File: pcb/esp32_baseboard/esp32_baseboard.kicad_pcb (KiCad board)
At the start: 2 copper layers, 175 x 175 mm, 38 parts, among them J1 Screw_12V_IN, J10 LIM_MIN_NC, J11 LIM_MAX_NC, J12 LIM_MIN_NC, J13 LIM_MAX_NC, J14 BUP_30S, J15 BUZZER_5V, J16 AOD4184, J17 TFT_TOUCH, J2 NEMA17_OUT, J4 OPTO_FIELD_IN, J5 GA12_N20, J6 GA12_N20, J7 GA12_N20, J8 LIM_MIN_NC, J9 LIM_MAX_NC, U1 ESP32_S3_DevKitC_1, U2 MP1584_5V3A, U3 TMC2209, U4 PC817_4CH, U5 DRV8871_Module, U6 DRV8871_Module, U7 DRV8871_Module, U8 MP1584_BLW, U9 PC817_4CH

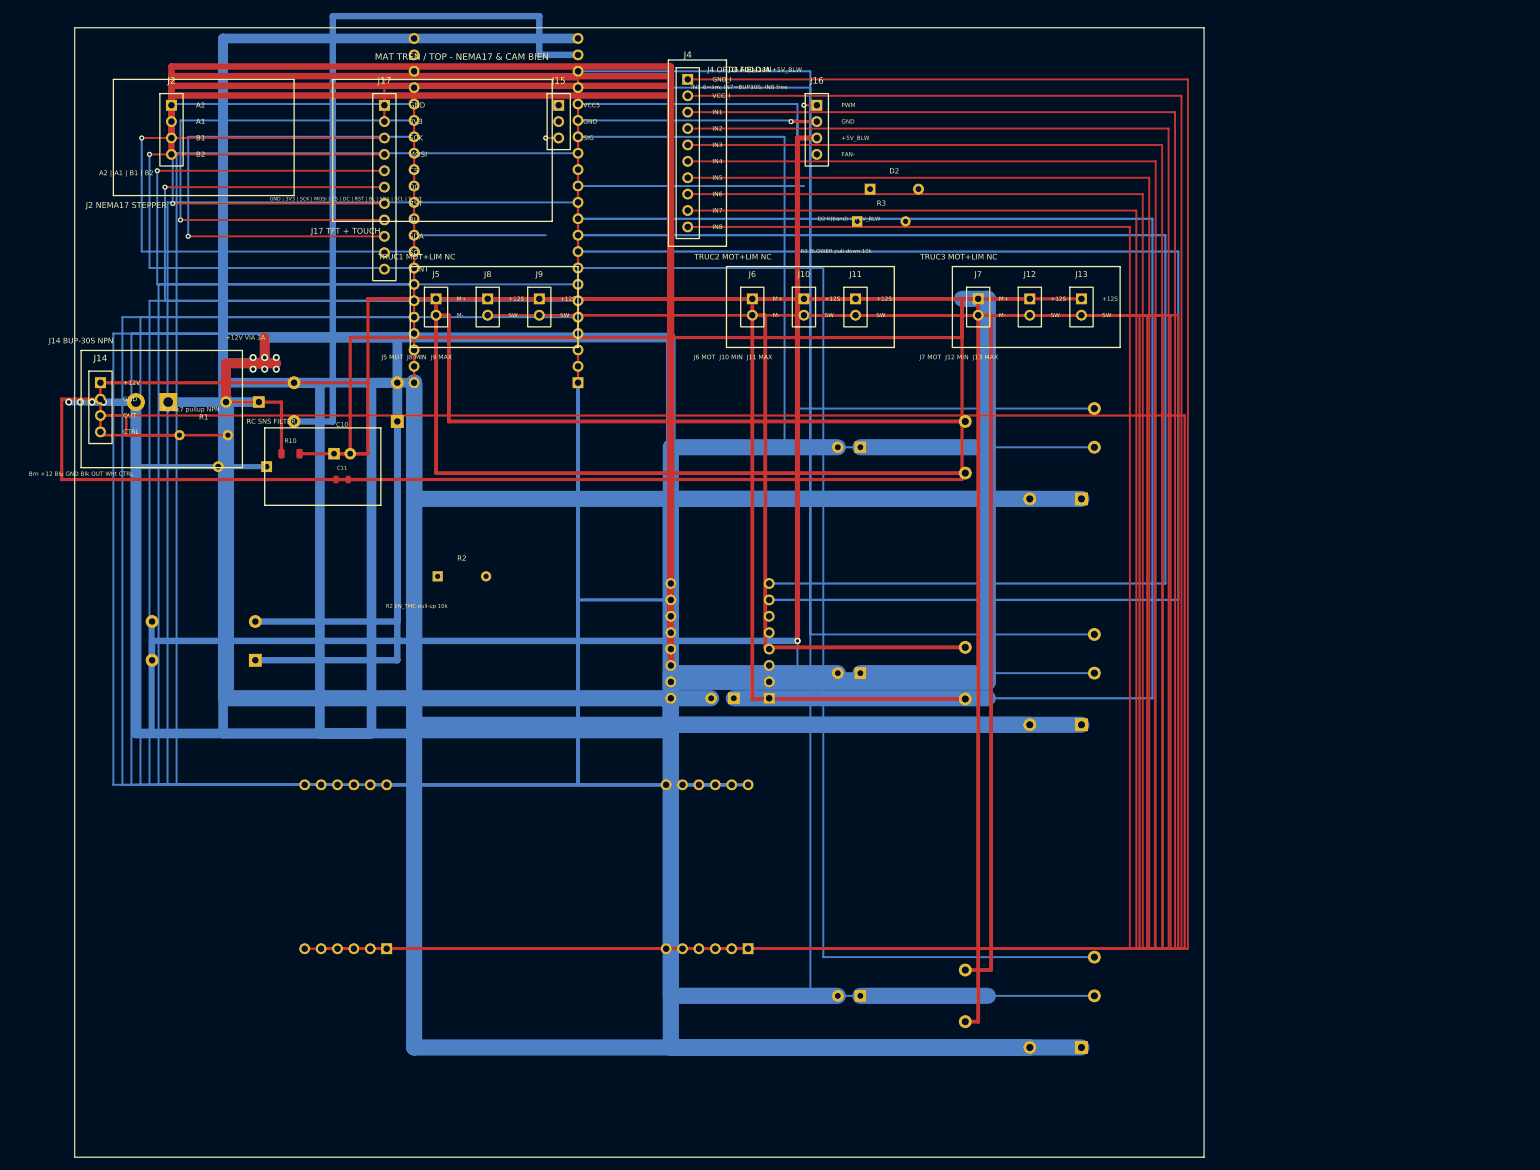
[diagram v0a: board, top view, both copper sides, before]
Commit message: sửa lỗi ngắn mạch trên board
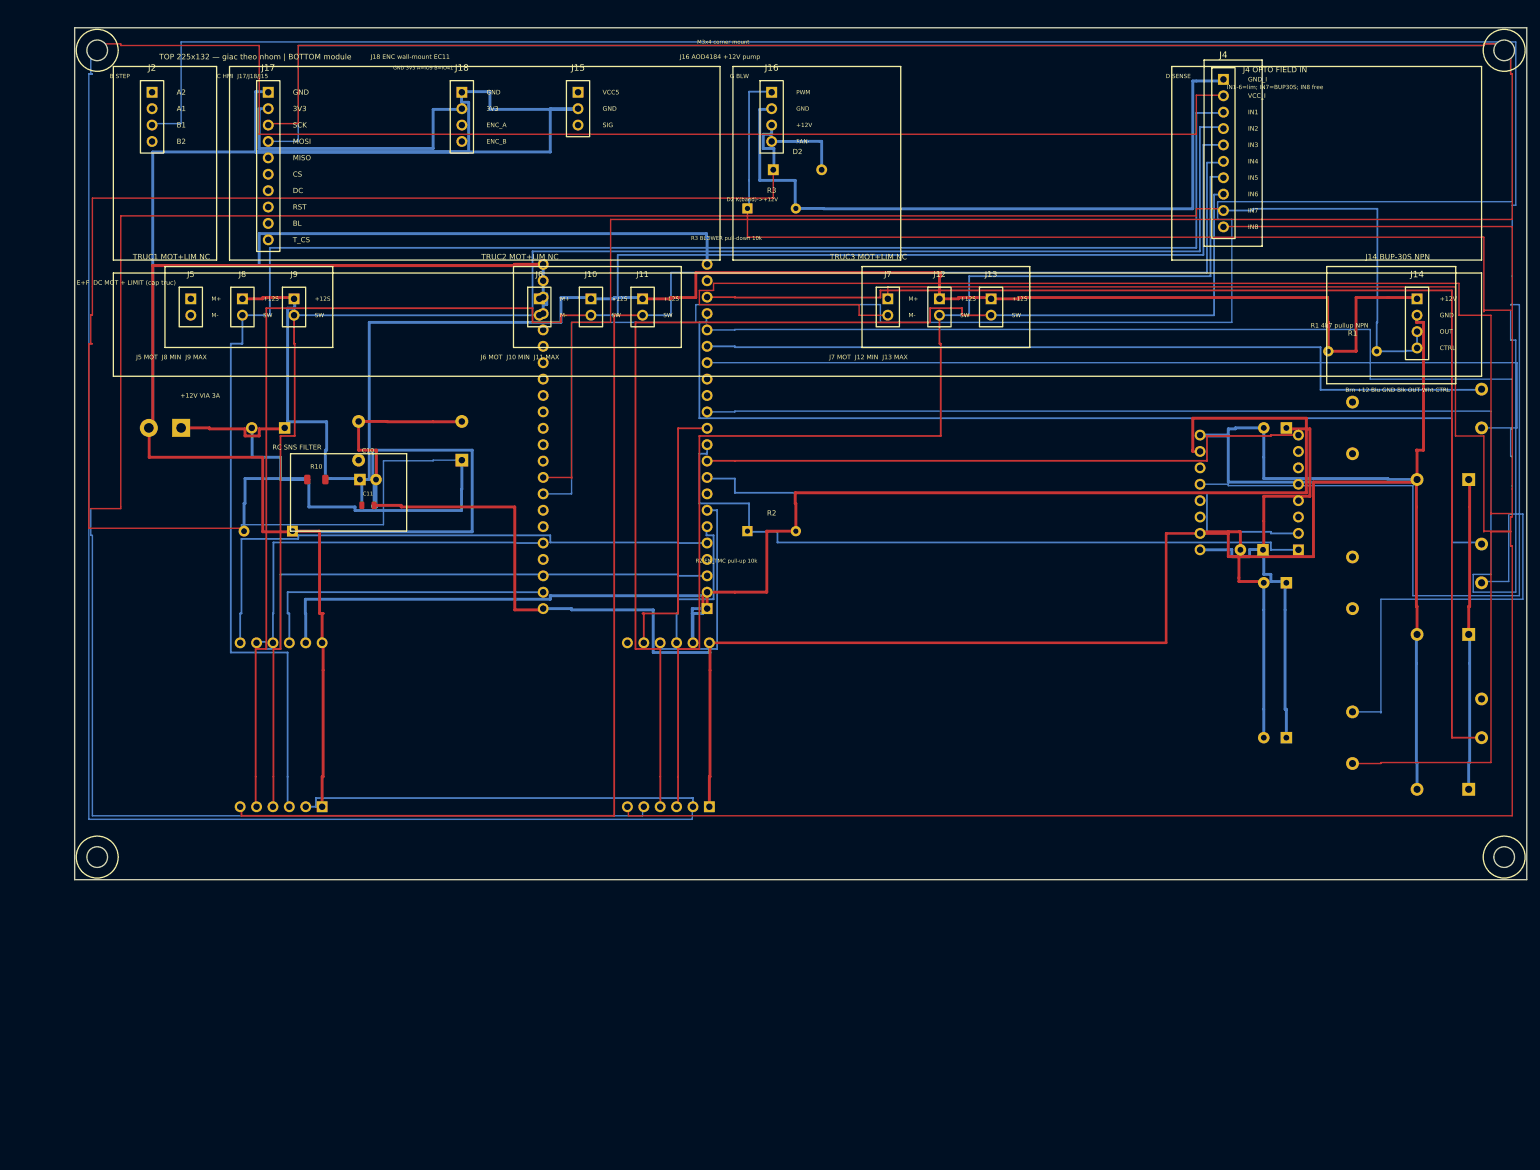
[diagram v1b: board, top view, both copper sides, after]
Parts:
- removed U8: MP1584_BLW, ESP32_Carrier:MP1584_5V3A
- added H1: M3, ESP32_Carrier:MountingHole_M3, F.Cu at (38.5, 33.5)
- added H2: M3, ESP32_Carrier:MountingHole_M3, F.Cu at (256.5, 33.5)
- added H3: M3, ESP32_Carrier:MountingHole_M3, F.Cu at (38.5, 158.5)
- added H4: M3, ESP32_Carrier:MountingHole_M3, F.Cu at (256.5, 158.5)
- added J18: EC11_ENC, ESP32_Carrier:PinHeader_1x04_ENC, F.Cu at (95.0, 40.0)
- J17: footprint ESP32_Carrier:PinHeader_1x11_TFT -> ESP32_Carrier:PinHeader_1x10_TFT
- moved J14 204.4 mm to (243.0, 72.0)
- moved R1 178.5 mm to (233.0, 80.1)
- moved U3 85.2 mm to (217.0, 102.0)
- moved C20 85.2 mm to (217.4, 110.9)
- moved J4 83.0 mm to (213.0, 38.0)
- moved C23 77.2 mm to (221.0, 140.0)
- moved U7 72.1 mm to (243.0, 140.0)
- moved C22 67.5 mm to (221.0, 116.0)
- moved C21 66.1 mm to (221.0, 92.0)
- moved U6 61.6 mm to (243.0, 116.0)
- moved U5 60.1 mm to (243.0, 92.0)
- moved R2 48.5 mm to (143.0, 108.0)
- moved U1 40.3 mm to (133.0, 120.0)
- moved J5 38.0 mm to (53.0, 72.0)
- moved J8 38.0 mm to (61.0, 72.0)
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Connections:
- net /I2C_SCL renamed /T_CS
- D2 pad 1: +5V_BLW -> +12V
- J16 pad 3: +5V_BLW -> +12V
- J17 pad 5: /TFT_CS -> /TFT_MISO
- J17 pad 6: /TFT_DC -> /TFT_CS
- J17 pad 7: /TFT_RST -> /TFT_DC
- J17 pad 8: /TFT_BL -> /TFT_RST
- J17 pad 9: /I2C_SDA -> /TFT_BL
- U1 pad 15: /OPTO_OUT8 -> /ENC_A
- U1 pad 29: /TP_INT -> /ENC_B
- U1 pad 39: /I2C_SDA -> /TFT_MISO
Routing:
- net GND: track 2326.1 -> 1179.7 mm, vias 5 -> 0
- net +12V: track 866.3 -> 435.4 mm, vias 6 -> 0
- net /OPTO_IN2: track 655.4 -> 253.0 mm, vias 1 -> 0
- net /OPTO_IN1: track 665.2 -> 270.5 mm, vias 1 -> 0
- net /OPTO_IN3: track 612.5 -> 257.1 mm, vias 1 -> 0
- net /OPTO_IN4: track 602.7 -> 255.2 mm, vias 1 -> 0
- net /TFT_MOSI: track 95.0 -> 437.6 mm, vias 1 -> 0
- net /TFT_SCK: track 97.4 -> 423.0 mm, vias 1 -> 0
- net /BLOWER: track 37.0 -> 359.9 mm, vias 1 -> 0
- net /OPTO_IN5: track 441.5 -> 182.9 mm, vias 1 -> 0
- net /OPTO_IN6: track 431.6 -> 192.1 mm, vias 1 -> 0
- net /OPTO_OUT8: track 235.9 -> 0.00 mm
- net +12V_SNS: track 487.6 -> 273.2 mm
- net /MotB1: track 170.2 -> 378.9 mm
- net /OPTO_OUT5: track 229.1 -> 24.9 mm
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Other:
- board size 175 x 175 mm -> 225 x 132 mm
- board text added: "1 POWER J1/U2"
- board text added: "2 MCU U1"
- board text added: "3 TMC"
- board text added: "B STEP"
- board text added: "B.Cu bus"
- board text added: "BOTTOM — 1 POWER | 2 MCU | 3 TMC | 4 OPTO | 5 DRV"
- board text added: "C HMI J17/J18/J15"
- board text added: "D SENSE"
- board text added: "D2 K(band)->+12V"
- board text added: "E+F DC MOT + LIMIT (cap truc)"
- board text added: "G BLW"
- board text added: "GND 3V3 A=IO9 B=IO41"
- board text added: "J16 AOD4184 +12V pump"
- board text added: "J18 ENC wall-mount EC11"
- board text added: "M3x4 corner mount"
- board text added: "TOP 225x132 — giac theo nhom | BOTTOM module"
- board text removed: "12V -> 5V logic"
- board text removed: "A2 | A1 | B1 | B2"
- board text removed: "AOD4184 / blower only"
- board text removed: "D2 K(band)->+5V_BLW"
- board text removed: "GND | 3V3 | SCK | MOSI | CS | DC | RST | BL | SDA | SCL | T_INT"
- board text removed: "J1 NGUON 12V-3A"
- board text removed: "J16 AOD4184 +5V_BLW"
- board text removed: "J17 TFT + TOUCH"
- board text removed: "J2 NEMA17 STEPPER"
- board text removed: "MAT DUOI / BOTTOM - MODULE ROI"
- board text removed: "MAT TREN / TOP - NEMA17 & CAM BIEN"
- board text removed: "U1 ESP32 DevKit V1"
- board text removed: "U2 MP1584EN LOGIC 5V"
- board text removed: "U3 TMC2209"
- board text removed: "U8 MP1584 +5V_BLW"
- board text removed: "stepstick NEMA17"
- board text removed: "via farm 6x0.6mm >=3A"
